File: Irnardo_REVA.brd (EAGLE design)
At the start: 12 x 17 mm, 20 parts, among them J1 USB_PAD, Q1 FA-20H, U1 ATMEGA32U4-MU, U2 TSOP755

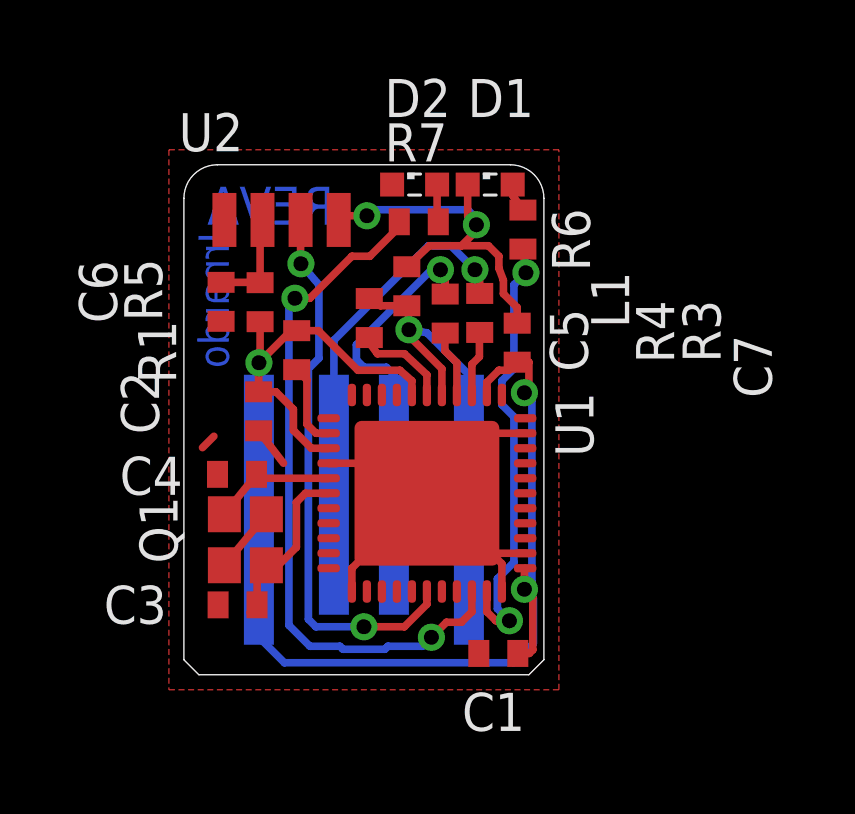
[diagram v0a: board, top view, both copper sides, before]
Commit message: Move a trace a little
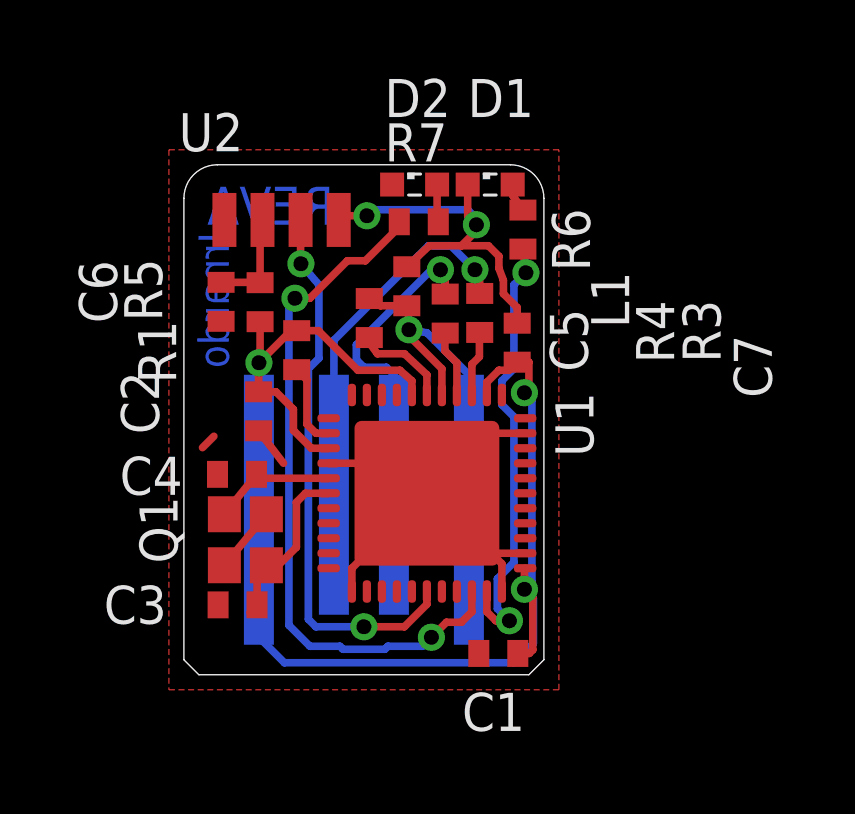
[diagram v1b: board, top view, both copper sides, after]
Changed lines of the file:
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@@
 <layer number="24" name="bOrigins" color="15" fill="1" visible="yes" active="yes"/>
 <layer number="25" name="tNames" color="7" fill="1" visible="yes" active="yes"/>
-<layer number="26" name="bNames" color="7" fill="1" visible="no" active="yes"/>
+<layer number="26" name="bNames" color="7" fill="1" visible="yes" active="yes"/>
 <layer number="27" name="tValues" color="7" fill="1" visible="no" active="yes"/>
 <layer number="28" name="bValues" color="7" fill="1" visible="no" active="yes"/>
@@
 <layer number="49" name="Reference" color="7" fill="1" visible="no" active="yes"/>
 <layer number="50" name="ReferenceLS" color="7" fill="1" visible="no" active="no"/>
-<layer number="51" name="tDocu" color="7" fill="1" visible="no" active="yes"/>
-<layer number="52" name="bDocu" color="7" fill="1" visible="no" active="yes"/>
+<layer number="51" name="tDocu" color="7" fill="1" visible="yes" active="yes"/>
+<layer number="52" name="bDocu" color="7" fill="1" visible="yes" active="yes"/>
 <layer number="53" name="tGND_GNDA" color="7" fill="1" visible="no" active="no"/>
 <layer number="54" name="bGND_GNDA" color="7" fill="1" visible="no" active="no"/>
@@
 <via x="8.25" y="1.25" extent="1-16" drill="0.5"/>
 <wire x1="7.18" y1="15.1" x2="7.18" y2="14.93" width="0.254" layer="1"/>
-<wire x1="7.18" y1="14.93" x2="6.2" y2="13.95" width="0.254" layer="1"/>
-<wire x1="6.2" y1="13.95" x2="5.6" y2="13.95" width="0.254" layer="1"/>
+<wire x1="7.18" y1="14.93" x2="6.05" y2="13.8" width="0.254" layer="1"/>
+<wire x1="6.05" y1="13.8" x2="5.45" y2="13.8" width="0.254" layer="1"/>
 <via x="3.7" y="12.55" extent="1-16" drill="0.5"/>
 <wire x1="3.7" y1="12.55" x2="3.5" y2="12.35" width="0.254" layer="16"/>
@@
 <wire x1="6.8" y1="0.95" x2="7.95" y2="0.95" width="0.254" layer="16"/>
 <wire x1="7.95" y1="0.95" x2="8.25" y2="1.25" width="0.254" layer="16"/>
-<wire x1="5.6" y1="13.95" x2="4.2" y2="12.55" width="0.254" layer="1"/>
+<wire x1="5.45" y1="13.8" x2="4.2" y2="12.55" width="0.254" layer="1"/>
 <wire x1="4.2" y1="12.55" x2="3.7" y2="12.55" width="0.254" layer="1"/>
 </signal>
